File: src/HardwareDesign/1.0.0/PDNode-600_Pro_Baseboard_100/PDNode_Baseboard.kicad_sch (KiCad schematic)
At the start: 0 parts

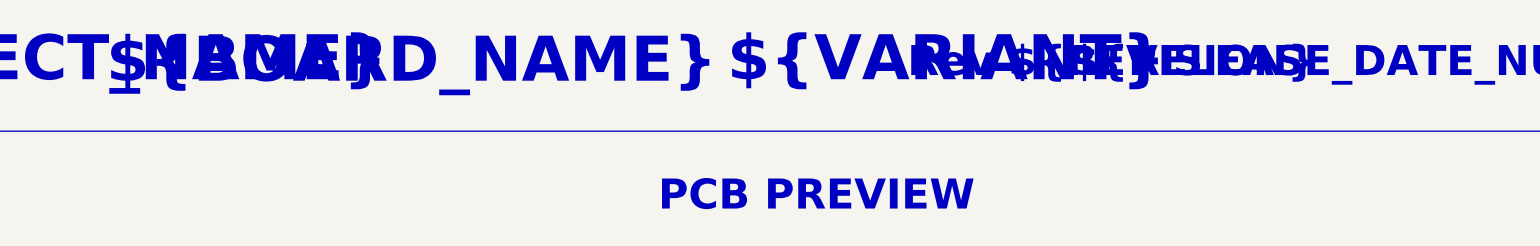
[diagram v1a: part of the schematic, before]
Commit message: baseboard development
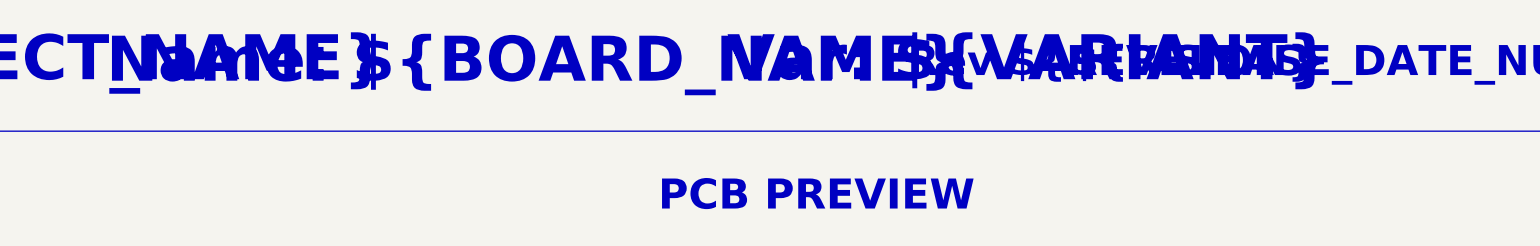
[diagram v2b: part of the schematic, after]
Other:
- note added: "Name: ${BOARD_NAME}"
- note added: "Var: ${VARIANT}"
- note removed: "${BOARD_NAME}"
- note removed: "${VARIANT}"
